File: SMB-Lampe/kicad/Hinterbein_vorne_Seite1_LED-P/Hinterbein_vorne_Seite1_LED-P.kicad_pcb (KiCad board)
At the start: 2 copper layers, 11.5 x 29.2 mm, 8 parts, among them J1 Conn_01x01_Pin, J2 Conn_01x01_Pin, J3 Conn_01x01_Pin

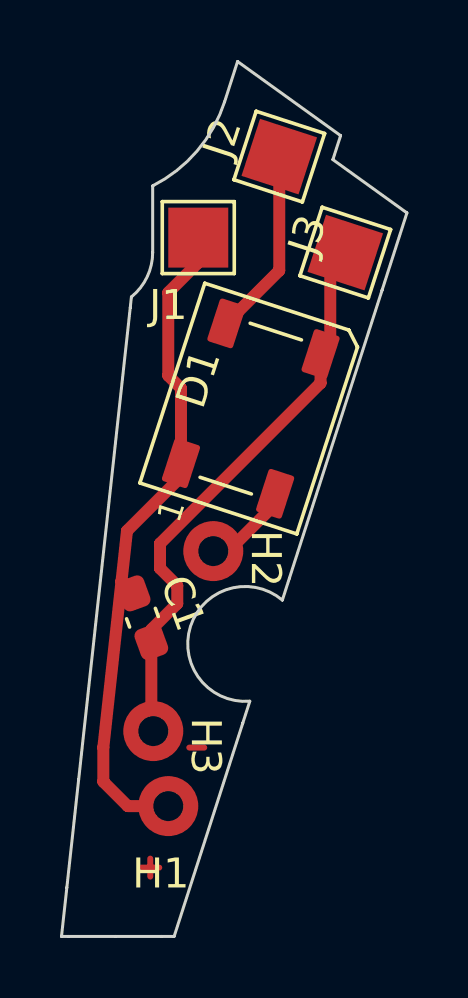
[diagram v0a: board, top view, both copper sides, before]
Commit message: Alle Platinen sind fertig zur Fertigung
Aus diesem Stand folgt das erste fertig leuchtende Pferd
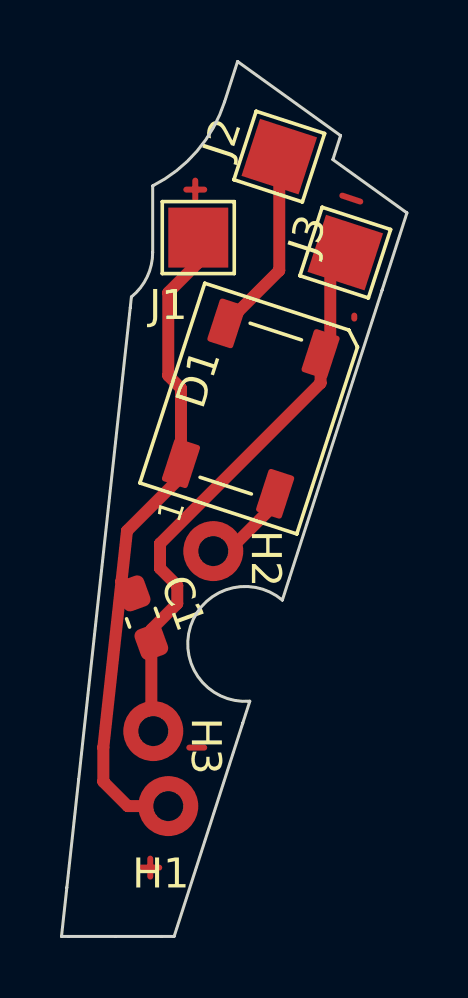
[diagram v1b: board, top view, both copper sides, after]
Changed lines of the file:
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@@
 		(tenting front back)
 		(pcbplotparams
-			(layerselection 0x00000000_00000000_55555555_57557573)
+			(layerselection 0x00000000_00000000_55555555_57555551)
 			(plot_on_all_layers_selection 0x00000000_00000000_00000000_00000000)
 			(disableapertmacros no)
@@
 	)
 	(gr_line
+		(start 149.9 63.9)
+		(end 149.9 64.5)
+		(stroke
+			(width 0.2)
+			(type default)
+		)
+		(layer "F.Cu")
+	)
+	(gr_line
+		(start 154.8 64.4)
+		(end 155.4 64.6)
+		(stroke
+			(width 0.2)
+			(type default)
+		)
+		(layer "F.Cu")
+	)
+	(gr_line
+		(start 155.2 68.4)
+		(end 155.2 68.5)
+		(stroke
+			(width 0.2)
+			(type default)
+		)
+		(layer "F.Cu")
+	)
+	(gr_line
+		(start 149.6 64.2)
+		(end 150.2 64.2)
+		(stroke
+			(width 0.2)
+			(type default)
+		)
+		(layer "F.Cu")
+	)
+	(gr_line
